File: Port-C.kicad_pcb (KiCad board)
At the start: 2 copper layers, 25 x 15 mm, 10 parts, among them J1 USB_C_Receptacle_USB2.0_14P, J2 Conn_01x04_Socket, U1 USBLC6-2SC6

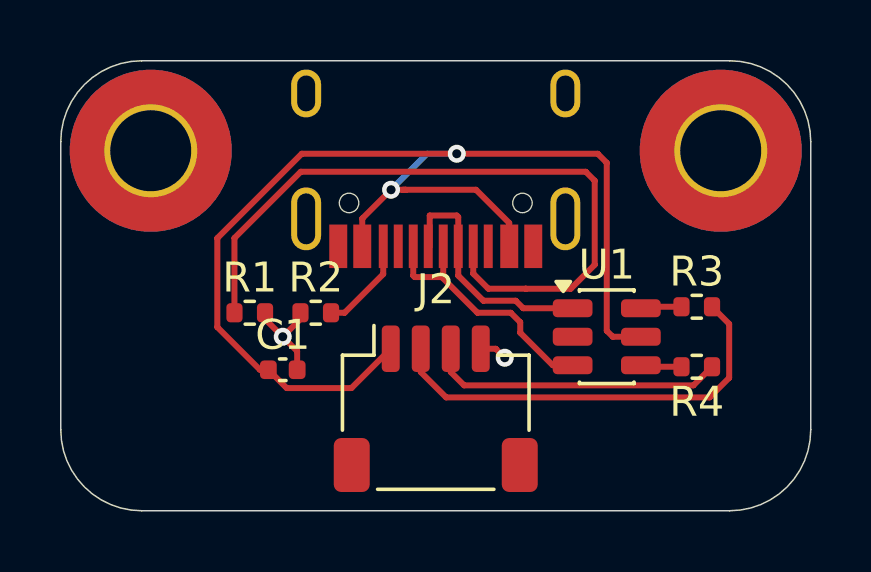
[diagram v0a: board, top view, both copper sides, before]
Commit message: Updated Files
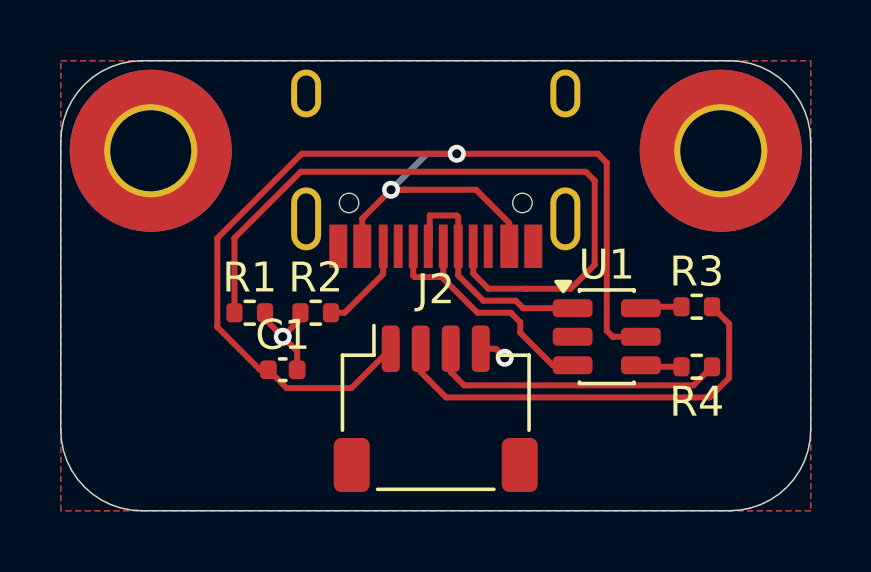
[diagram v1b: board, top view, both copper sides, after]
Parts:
- H1, H2: moved to B.Cu
- turned H1 to 180 degrees
- turned H2 to 180 degrees
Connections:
- J2 pad 1: +5V -> VBUS
- R3 pad 2: USB_D- -> USB_D+
- R4 pad 1: USB_D+ -> USB_D-
- U1 pad 1: USB_D- -> USB_D+
- U1 pad 3: USB_D+ -> USB_D-
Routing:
- added copper zone on B.Cu, net GND
- added copper zone on F.Cu, net GND
